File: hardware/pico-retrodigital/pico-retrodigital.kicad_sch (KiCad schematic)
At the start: 50 parts, among them J1 Conn_02x05_Top_Bottom, J2 HDMI_A, J3 Conn_01x03, J4 Conn_01x02_Pin, J5 USB_C, SW1 SW_Push, U1 74LVC2G17, U2 74LVC2G17, U3 SN74LVC8T245, U4 SN74LVC8T245, U5 74LVC2G17, U6 74LVC2G17, U7 RP2350B, U8 NCP1117-3.3_SOT223, Y1 ABM8-272-T3

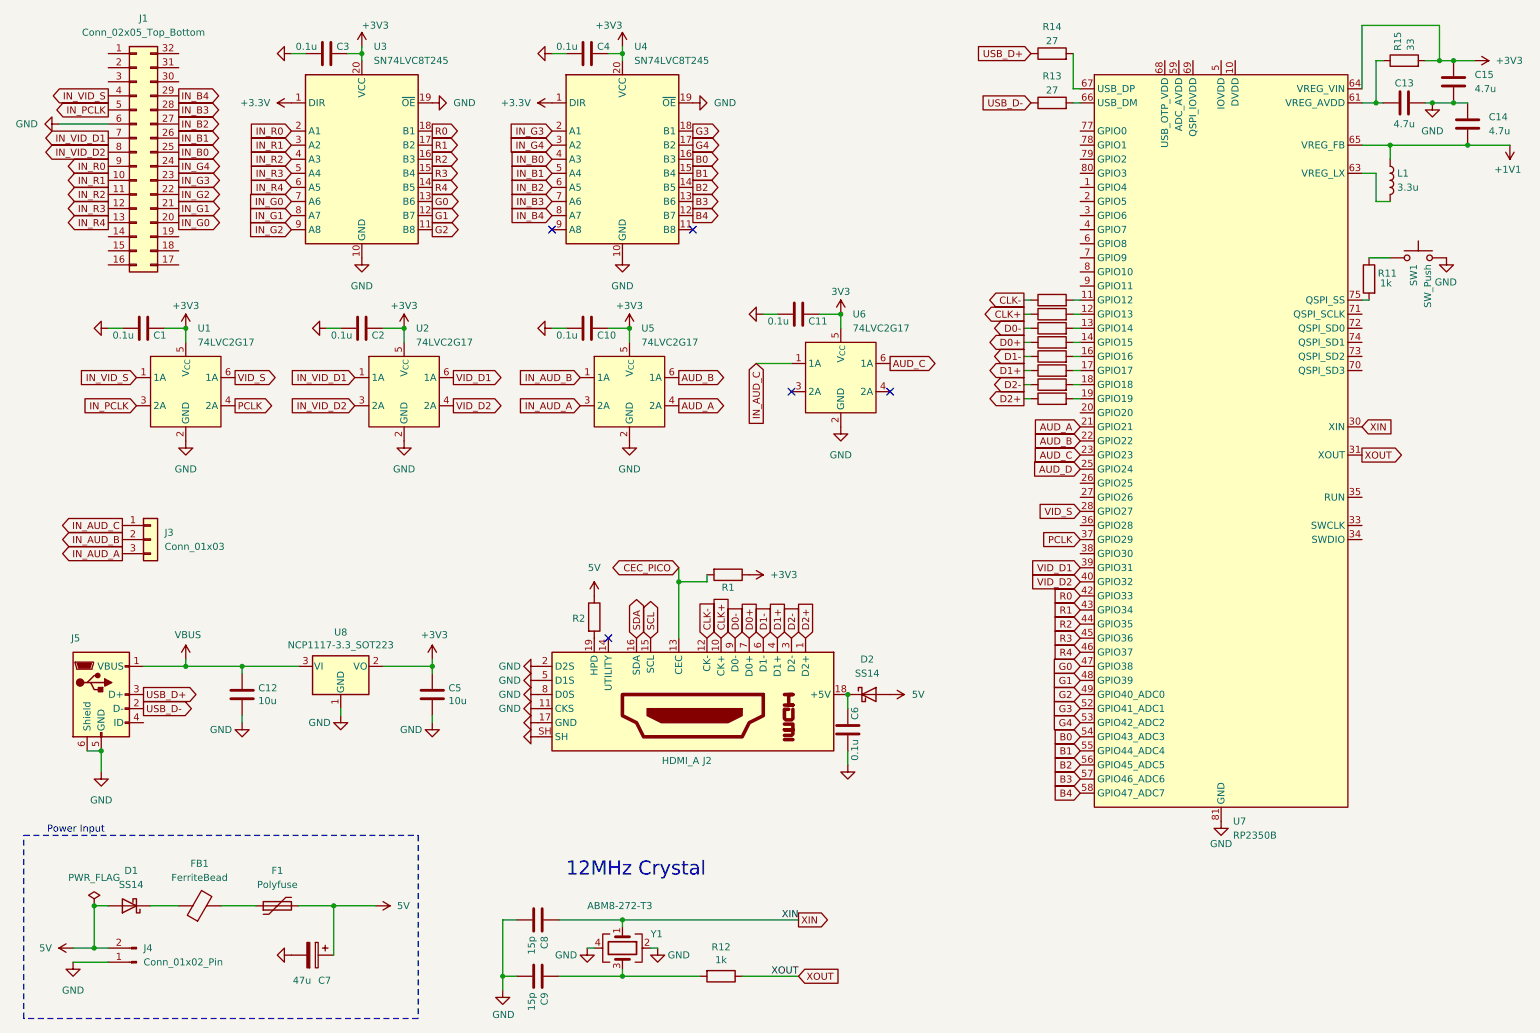
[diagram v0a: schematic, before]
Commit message: Update hardware
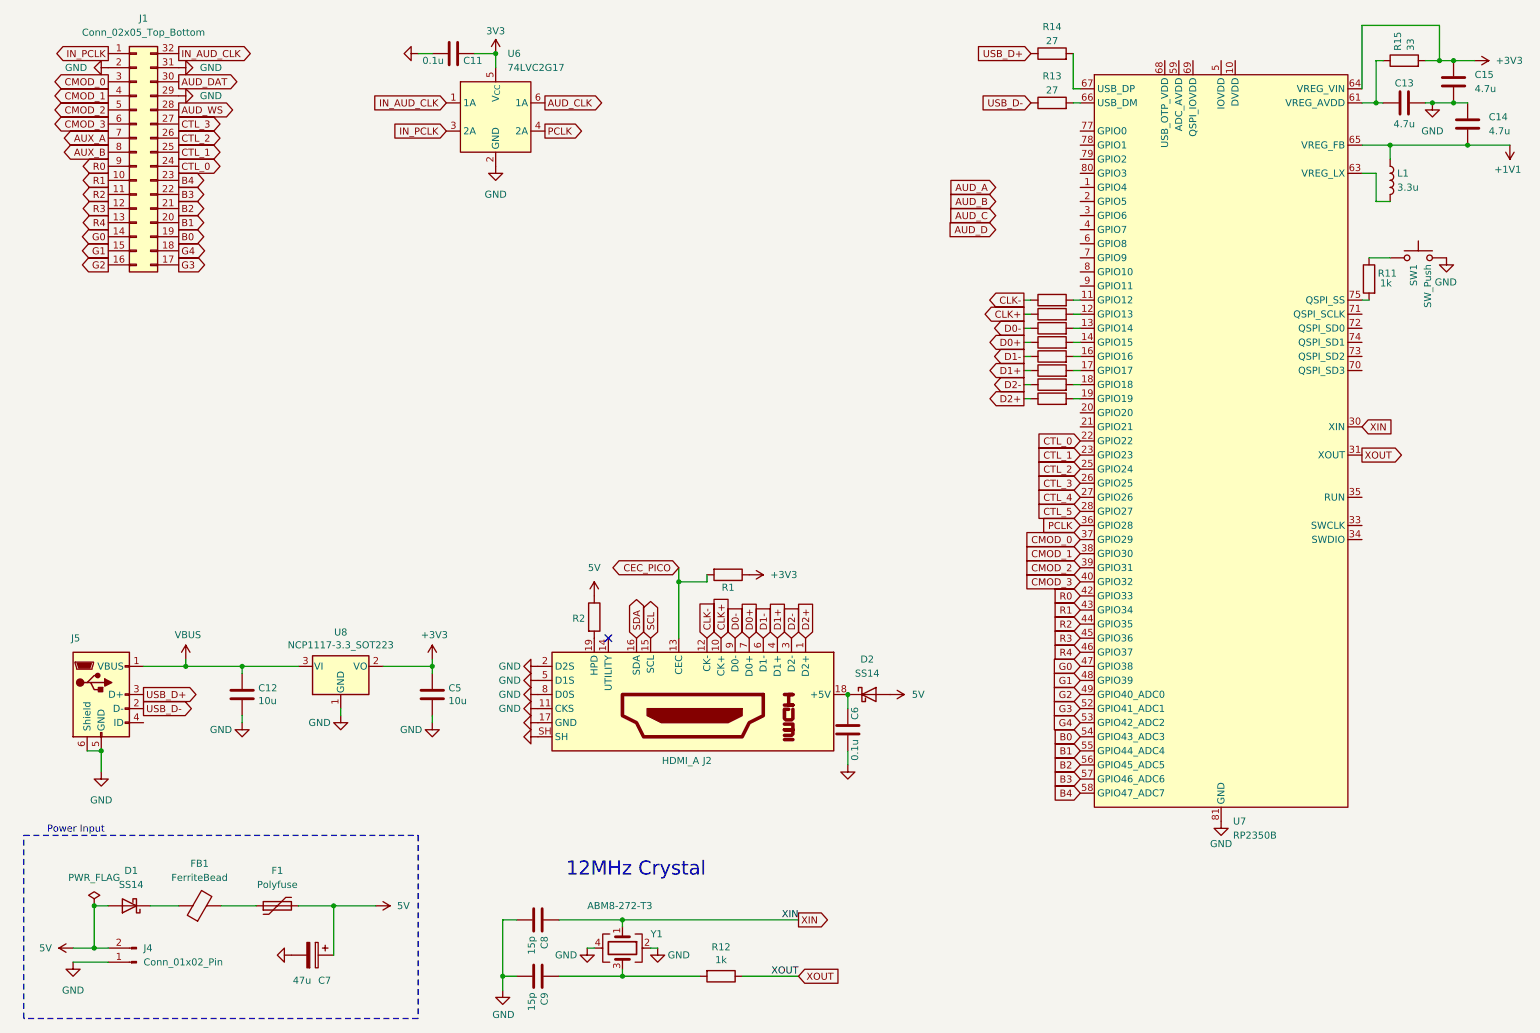
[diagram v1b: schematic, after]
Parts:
- removed C1, C10, C2, C3, C4: 0.1u, Capacitor_SMD:C_0603_1608Metric, symbol Device:C
- removed J3: Conn_01x03, Connector_PinHeader_2.54mm:PinHeader_1x03_P2.54mm_Vertical, symbol Connector_Generic:Conn_01x03
- removed U1, U2, U5: 74LVC2G17, Package_TO_SOT_SMD:SOT-23-6, symbol pico-retrodigital:74LVC2G17_SINGLE
- removed U3, U4: SN74LVC8T245, custom_components:TSSOP-20_4.4x6.5mm_Pitch0.65mm_Handsoldering, symbol Logic_LevelTranslator:SN74LVC245APW
- J1: footprint Connector_FFC-FPC:TE_2-1734839-0_1x20-1MP_P0.5mm_Horizontal -> Connector_FFC-FPC:TE_3-1734839-2_1x32-1MP_P0.5mm_Horizontal
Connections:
- net IN_AUD_C is gone; now on net IN_AUD_CLK: U6.1 (1A)
- net IN_B2 is gone; now on net CTL_3: J1.27 (Pin_27)
- net IN_B4 is gone; now on net GND: J1.29 (Pin_29)
- net IN_G0 is gone; now on net B1: J1.20 (Pin_20)
- net IN_G1 is gone; now on net B2: J1.21 (Pin_21)
- net IN_G2 is gone; now on net B3: J1.22 (Pin_22)
- net IN_G3 is gone; now on net B4: J1.23 (Pin_23)
- net IN_R0 is gone; now on net R0: J1.9 (Pin_9)
- net IN_R1 is gone; now on net R1: J1.10 (Pin_10)
- net IN_R2 is gone; now on net R2: J1.11 (Pin_11)
- net IN_R3 is gone; now on net R3: J1.12 (Pin_12)
- net IN_R4 is gone; now on net R4: J1.13 (Pin_13)
- net IN_VID_S is gone; now on net CMOD_1: J1.4 (Pin_4)
- net AUD_A: no longer U7.21 (GPIO21)
- net AUD_B: no longer U7.22 (GPIO22)
- net AUD_C: no longer U6.6 (1A), U7.23 (GPIO23)
- net AUD_D: no longer U7.25 (GPIO24)
- net B0: now also J1.19 (Pin_19)
- net G0: now also J1.14 (Pin_14)
- net G1: now also J1.15 (Pin_15)
- net G2: now also J1.16 (Pin_16)
- net G3: now also J1.17 (Pin_17)
- net G4: now also J1.18 (Pin_18)
- net GND: now also J1.2 (Pin_2), J1.31 (Pin_31); no longer J1.6 (Pin_6)
- net IN_PCLK: now also J1.1 (Pin_1), U6.3 (2A); no longer J1.5 (Pin_5)
- net PCLK: now also U6.4 (2A), U7.36 (GPIO28); no longer U7.37 (GPIO29)
- net CMOD_0: now reaches J1.3 (Pin_3)
- net CMOD_0: now also U7.37 (GPIO29)
- net AUD_DAT: now reaches J1.30 (Pin_30)
- net IN_AUD_CLK: now reaches J1.32 (Pin_32)
- net CTL_3: now reaches U7.26 (GPIO25)
- net CTL_4: now reaches U7.27 (GPIO26)
- net CMOD_1: now reaches U7.38 (GPIO30)
- net IN_B0 renamed CTL_1
- net CTL_1: now also U7.23 (GPIO23)
- net IN_B1 renamed CTL_2
- net CTL_2: now also U7.25 (GPIO24)
- net IN_B3 renamed AUD_WS
- net IN_G4 renamed CTL_0
- net CTL_0: now also U7.22 (GPIO22)
- net IN_VID_D1 renamed AUX_A
- net IN_VID_D2 renamed AUX_B
- net VID_D1 renamed CMOD_2
- net CMOD_2: now also J1.5 (Pin_5)
- net VID_D2 renamed CMOD_3
- net CMOD_3: now also J1.6 (Pin_6)
- net VID_S renamed CTL_5
- new net AUD_CLK: U6.6 (1A)
- no-connect marks 5 -> 1
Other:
- moved on the sheet: C11, U6
